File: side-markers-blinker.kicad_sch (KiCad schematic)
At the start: 35 parts, among them J1 Conn_01x04_Socket, J2 Conn_01x02_Socket, J3 Conn_01x04_Socket, J4 Conn_01x02_Socket, Q1 IRF540N, Q2 BC546, Q3 BC546, Q4 IRF540N, Q5 BC546, Q6 BC546

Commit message: Reduce board size.
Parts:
- D1, D10, D2, D3, D4, D5, D6, D7, D8, D9: footprint Diode_THT:D_5W_P12.70mm_Horizontal -> Diode_THT:D_DO-41_SOD81_P7.62mm_Horizontal
- R1, R10, R11, R12, R2, R3, R4, R5, R6, R7, R8, R9: footprint Resistor_THT:R_Axial_DIN0411_L9.9mm_D3.6mm_P20.32mm_Horizontal -> Resistor_THT:R_Axial_DIN0207_L6.3mm_D2.5mm_P7.62mm_Horizontal
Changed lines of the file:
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@@
       (effects (font (size 1.27 1.27)) (justify right))
     )
-    (property "Footprint" "Diode_THT:D_5W_P12.70mm_Horizontal" (at 123.19 33.02 90)
+    (property "Footprint" "Diode_THT:D_DO-41_SOD81_P7.62mm_Horizontal" (at 123.19 33.02 90)
       (effects (font (size 1.27 1.27)) hide)
     )
@@
       (effects (font (size 1.27 1.27)))
     )
-    (property "Footprint" "Resistor_THT:R_Axial_DIN0411_L9.9mm_D3.6mm_P20.32mm_Horizontal" (at 114.3 27.94 0)
+    (property "Footprint" "Resistor_THT:R_Axial_DIN0207_L6.3mm_D2.5mm_P7.62mm_Horizontal" (at 114.3 27.94 0)
       (effects (font (size 1.27 1.27)) hide)
     )
@@
       (effects (font (size 1.27 1.27)))
     )
-    (property "Footprint" "Resistor_THT:R_Axial_DIN0411_L9.9mm_D3.6mm_P20.32mm_Horizontal" (at 119.38 115.57 0)
+    (property "Footprint" "Resistor_THT:R_Axial_DIN0207_L6.3mm_D2.5mm_P7.62mm_Horizontal" (at 119.38 115.57 0)
       (effects (font (size 1.27 1.27)) hide)
     )
@@
       (effects (font (size 1.27 1.27)))
     )
-    (property "Footprint" "Resistor_THT:R_Axial_DIN0411_L9.9mm_D3.6mm_P20.32mm_Horizontal" (at 135.89 102.87 0)
+    (property "Footprint" "Resistor_THT:R_Axial_DIN0207_L6.3mm_D2.5mm_P7.62mm_Horizontal" (at 135.89 102.87 0)
       (effects (font (size 1.27 1.27)) hide)
     )
@@
       (effects (font (size 1.27 1.27)))
     )
-    (property "Footprint" "Resistor_THT:R_Axial_DIN0411_L9.9mm_D3.6mm_P20.32mm_Horizontal" (at 116.84 50.8 0)
+    (property "Footprint" "Resistor_THT:R_Axial_DIN0207_L6.3mm_D2.5mm_P7.62mm_Horizontal" (at 116.84 50.8 0)
       (effects (font (size 1.27 1.27)) hide)
     )
@@
       (effects (font (size 1.27 1.27)) (justify right))
     )
-    (property "Footprint" "Diode_THT:D_5W_P12.70mm_Horizontal" (at 93.98 102.87 90)
+    (property "Footprint" "Diode_THT:D_DO-41_SOD81_P7.62mm_Horizontal" (at 93.98 102.87 90)
       (effects (font (size 1.27 1.27)) hide)
     )
@@
       (effects (font (size 1.27 1.27)) (justify right))
     )
-    (property "Footprint" "Diode_THT:D_5W_P12.70mm_Horizontal" (at 115.57 107.95 90)
+    (property "Footprint" "Diode_THT:D_DO-41_SOD81_P7.62mm_Horizontal" (at 115.57 107.95 90)
       (effects (font (size 1.27 1.27)) hide)
     )
@@
       (effects (font (size 1.27 1.27)))
     )
-    (property "Footprint" "Resistor_THT:R_Axial_DIN0411_L9.9mm_D3.6mm_P20.32mm_Horizontal" (at 60.96 170.18 0)
+    (property "Footprint" "Resistor_THT:R_Axial_DIN0207_L6.3mm_D2.5mm_P7.62mm_Horizontal" (at 60.96 170.18 0)
       (effects (font (size 1.27 1.27)) hide)
     )
@@
       (effects (font (size 1.27 1.27)))
     )
-    (property "Footprint" "Resistor_THT:R_Axial_DIN0411_L9.9mm_D3.6mm_P20.32mm_Horizontal" (at 99.06 38.1 0)
+    (property "Footprint" "Resistor_THT:R_Axial_DIN0207_L6.3mm_D2.5mm_P7.62mm_Horizontal" (at 99.06 38.1 0)
       (effects (font (size 1.27 1.27)) hide)
     )
@@
       (effects (font (size 1.27 1.27)))
     )
-    (property "Footprint" "Resistor_THT:R_Axial_DIN0411_L9.9mm_D3.6mm_P20.32mm_Horizontal" (at 60.96 156.21 0)
+    (property "Footprint" "Resistor_THT:R_Axial_DIN0207_L6.3mm_D2.5mm_P7.62mm_Horizontal" (at 60.96 156.21 0)
       (effects (font (size 1.27 1.27)) hide)
     )
@@
       (effects (font (size 1.27 1.27)) (justify left))
     )
-    (property "Footprint" "Resistor_THT:R_Axial_DIN0411_L9.9mm_D3.6mm_P20.32mm_Horizontal" (at 144.78 106.68 0)
+    (property "Footprint" "Resistor_THT:R_Axial_DIN0207_L6.3mm_D2.5mm_P7.62mm_Horizontal" (at 144.78 106.68 0)
       (effects (font (size 1.27 1.27)) hide)
     )
@@
       (effects (font (size 1.27 1.27)))
     )
-    (property "Footprint" "Resistor_THT:R_Axial_DIN0411_L9.9mm_D3.6mm_P20.32mm_Horizontal" (at 133.35 38.1 0)
+    (property "Footprint" "Resistor_THT:R_Axial_DIN0207_L6.3mm_D2.5mm_P7.62mm_Horizontal" (at 133.35 38.1 0)
       (effects (font (size 1.27 1.27)) hide)
     )
@@
       (effects (font (size 1.27 1.27)) (justify right))
     )
-    (property "Footprint" "Diode_THT:D_5W_P12.70mm_Horizontal" (at 91.44 38.1 90)
+    (property "Footprint" "Diode_THT:D_DO-41_SOD81_P7.62mm_Horizontal" (at 91.44 38.1 90)
       (effects (font (size 1.27 1.27)) hide)
     )
@@
       (effects (font (size 1.27 1.27)))
     )
-    (property "Footprint" "Diode_THT:D_5W_P12.70mm_Horizontal" (at 119.38 102.87 90)
+    (property "Footprint" "Diode_THT:D_DO-41_SOD81_P7.62mm_Horizontal" (at 119.38 102.87 90)
       (effects (font (size 1.27 1.27)) hide)
     )
@@
       (effects (font (size 1.27 1.27)))
     )
-    (property "Footprint" "Resistor_THT:R_Axial_DIN0411_L9.9mm_D3.6mm_P20.32mm_Horizontal" (at 101.6 102.87 0)
+    (property "Footprint" "Resistor_THT:R_Axial_DIN0207_L6.3mm_D2.5mm_P7.62mm_Horizontal" (at 101.6 102.87 0)
       (effects (font (size 1.27 1.27)) hide)
     )
@@
       (effects (font (size 1.27 1.27)))
     )
-    (property "Footprint" "Resistor_THT:R_Axial_DIN0411_L9.9mm_D3.6mm_P20.32mm_Horizontal" (at 116.84 92.71 0)
+    (property "Footprint" "Resistor_THT:R_Axial_DIN0207_L6.3mm_D2.5mm_P7.62mm_Horizontal" (at 116.84 92.71 0)
       (effects (font (size 1.27 1.27)) hide)
     )
@@
       (effects (font (size 1.27 1.27)) (justify right))
     )
-    (property "Footprint" "Diode_THT:D_5W_P12.70mm_Horizontal" (at 125.73 97.79 90)
+    (property "Footprint" "Diode_THT:D_DO-41_SOD81_P7.62mm_Horizontal" (at 125.73 97.79 90)
       (effects (font (size 1.27 1.27)) hide)
     )
@@
       (effects (font (size 1.27 1.27)) (justify right))
     )
-    (property "Footprint" "Diode_THT:D_5W_P12.70mm_Horizontal" (at 101.6 45.72 90)
+    (property "Footprint" "Diode_THT:D_DO-41_SOD81_P7.62mm_Horizontal" (at 101.6 45.72 90)
       (effects (font (size 1.27 1.27)) hide)
     )
@@
       (effects (font (size 1.27 1.27)) (justify right))
     )
-    (property "Footprint" "Diode_THT:D_5W_P12.70mm_Horizontal" (at 104.14 110.49 90)
+    (property "Footprint" "Diode_THT:D_DO-41_SOD81_P7.62mm_Horizontal" (at 104.14 110.49 90)
       (effects (font (size 1.27 1.27)) hide)
     )
@@
       (effects (font (size 1.27 1.27)) (justify left))
     )
-    (property "Footprint" "Resistor_THT:R_Axial_DIN0411_L9.9mm_D3.6mm_P20.32mm_Horizontal" (at 142.24 41.91 0)
+    (property "Footprint" "Resistor_THT:R_Axial_DIN0207_L6.3mm_D2.5mm_P7.62mm_Horizontal" (at 142.24 41.91 0)
       (effects (font (size 1.27 1.27)) hide)
     )
@@
       (effects (font (size 1.27 1.27)) (justify right))
     )
-    (property "Footprint" "Diode_THT:D_5W_P12.70mm_Horizontal" (at 113.03 43.18 90)
+    (property "Footprint" "Diode_THT:D_DO-41_SOD81_P7.62mm_Horizontal" (at 113.03 43.18 90)
       (effects (font (size 1.27 1.27)) hide)
     )
@@
       (effects (font (size 1.27 1.27)))
     )
-    (property "Footprint" "Diode_THT:D_5W_P12.70mm_Horizontal" (at 116.84 38.1 90)
-      (effects (font (size 1.27 1.27)) hide)
-    )
+    (property "Footprint" "Diode_THT:D_DO-41_SOD81_P7.62mm_Horizontal" (at 116.84 38.1 90)
+      (effects (font (size 1.27 1.27)) hide)
+    )

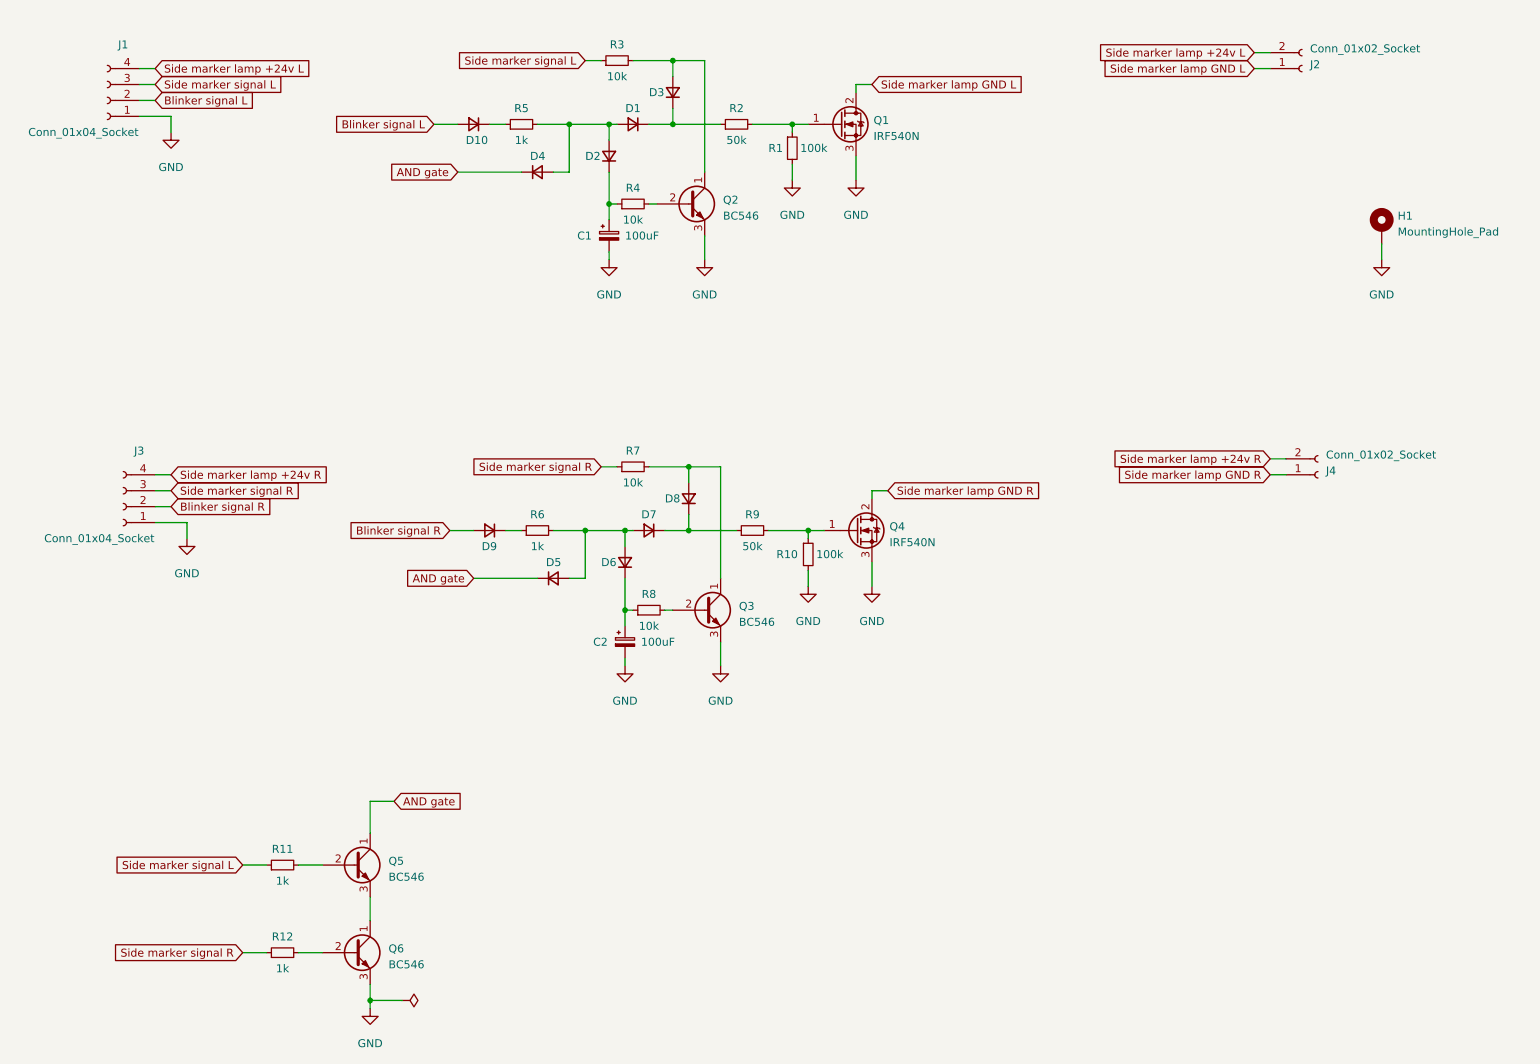
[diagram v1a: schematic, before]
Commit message: Remove unnecesary conections.
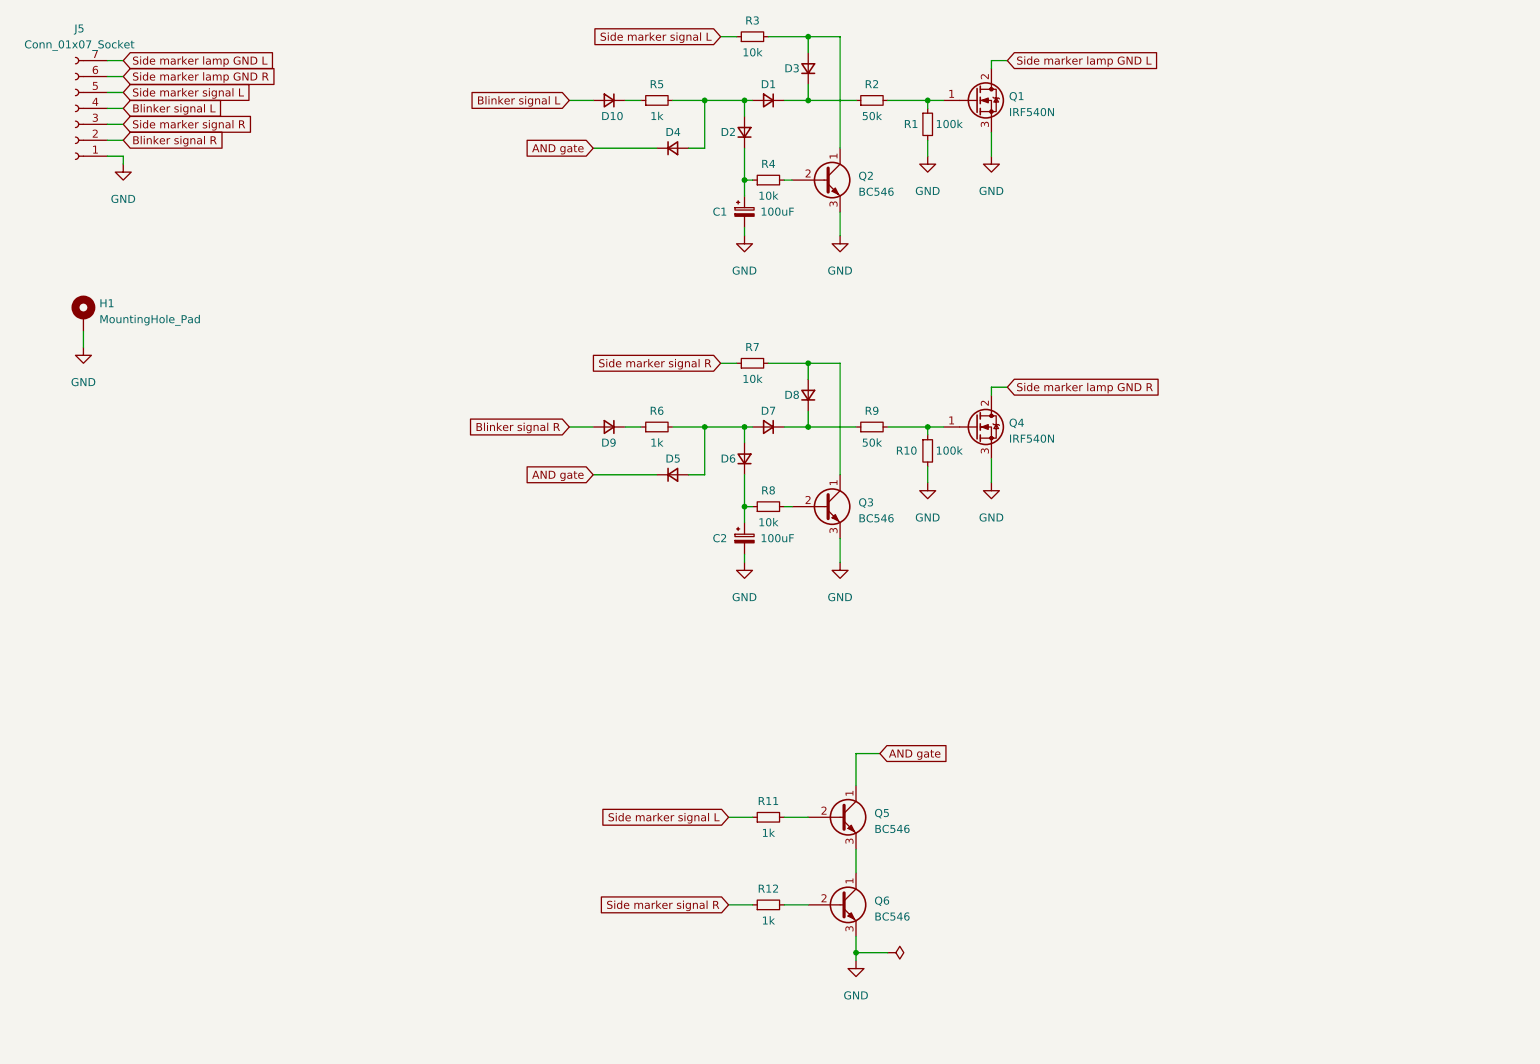
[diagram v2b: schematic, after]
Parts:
- removed J1, J3: Conn_01x04_Socket, Connector_Wire:SolderWire-2.5sqmm_1x04_P8.8mm_D2.4mm_OD4.4mm, symbol Connector:Conn_01x04_Socket
- removed J2, J4: Conn_01x02_Socket, Connector_Wire:SolderWire-2.5sqmm_1x02_P8.8mm_D2.4mm_OD4.4mm, symbol Connector:Conn_01x02_Socket
- added J5: Conn_01x07_Socket, Connector_TE-Connectivity:TE_826576-7_1x07_P3.96mm_Vertical, symbol Connector:Conn_01x07_Socket
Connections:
- net Blinker signal L: now also J5.4 (Pin_4)
- net Blinker signal R: now also J5.2 (Pin_2)
- net GND: now also J5.1 (Pin_1)
- net Side marker lamp GND L: now also J5.7 (Pin_7)
- net Side marker lamp GND R: now also J5.6 (Pin_6)
- net Side marker signal L: now also J5.5 (Pin_5)
- net Side marker signal R: now also J5.3 (Pin_3)
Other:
- moved on the sheet: C1, C2, D1, D10, D2, D3, D4, D5, D6, D7, D8, D9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
